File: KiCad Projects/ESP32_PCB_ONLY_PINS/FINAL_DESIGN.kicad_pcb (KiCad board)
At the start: 2 copper layers, 78 x 94.8 mm, 68 parts, among them J1 Screw_Terminal_01x02, J2 Conn_01x19_Socket, J3 Conn_01x19_Socket, J4 Conn_01x19_Socket, J5 Conn_01x19_Socket, Q1 PMOS, U1 LM2596S-5, U2 ESP32_NODEMCU

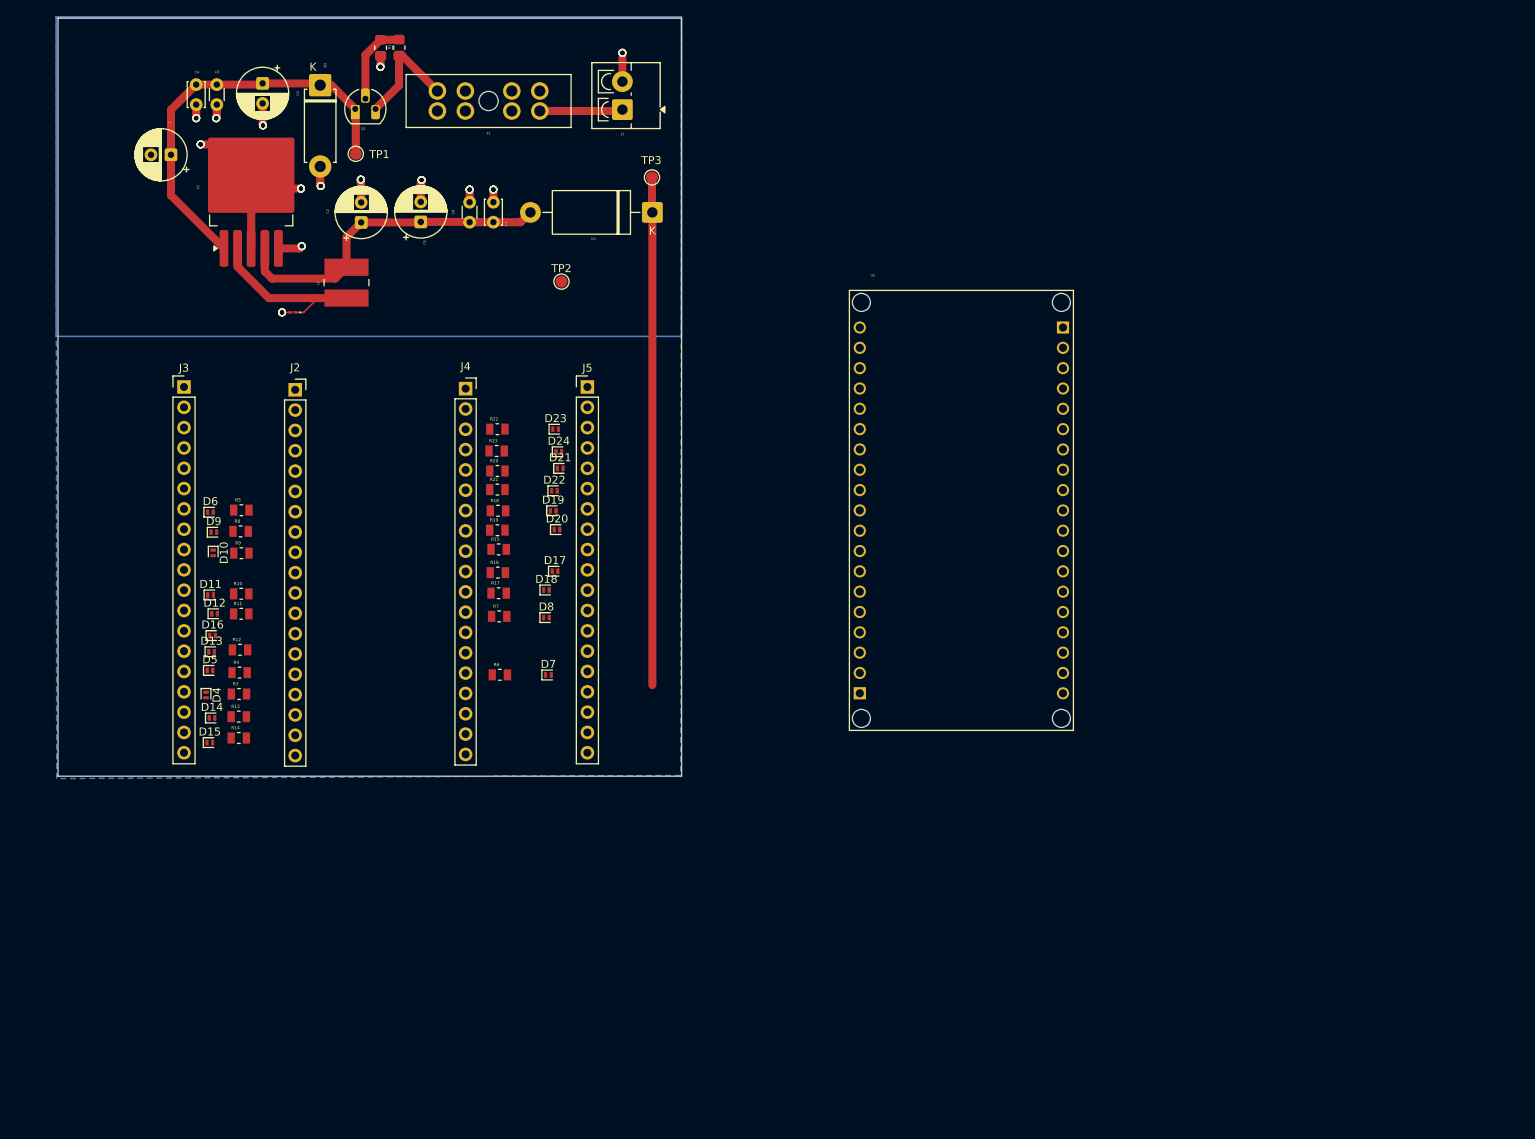
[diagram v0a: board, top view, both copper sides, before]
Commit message: PCB MODIFIED INSIDE ONLYPINS
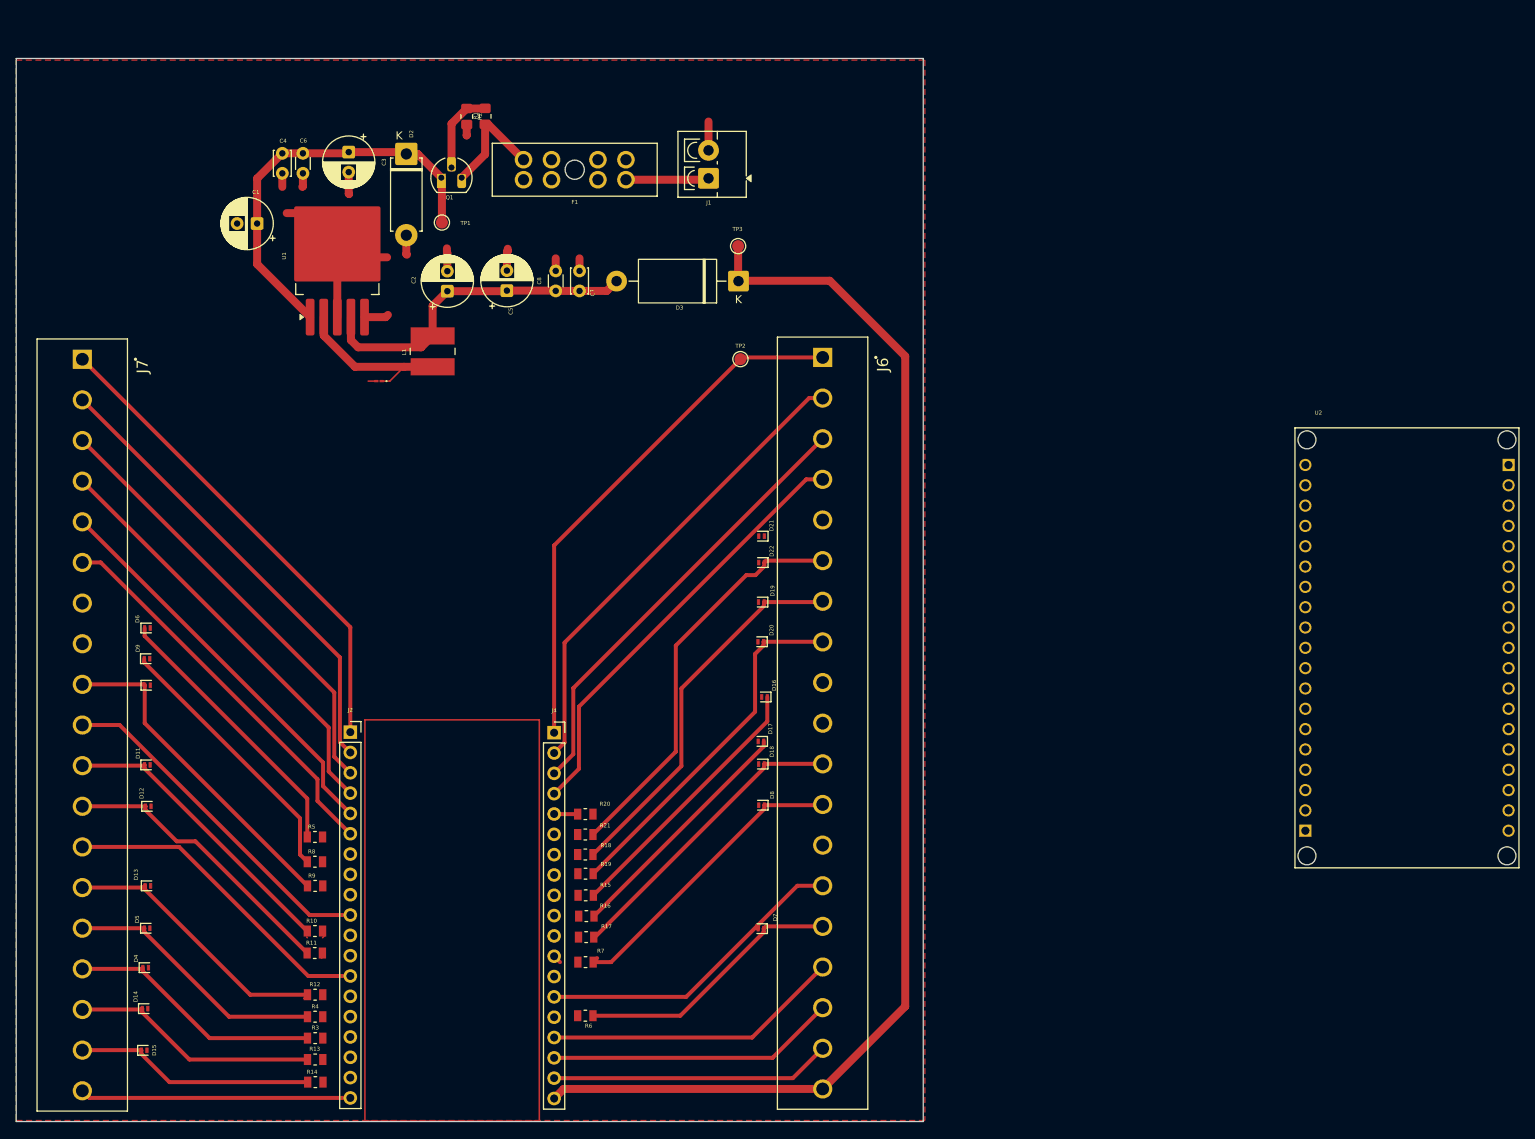
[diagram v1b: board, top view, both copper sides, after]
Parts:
- removed D23, D24: D_Zener, Diode_SMD:D_SOD-882
- removed J3, J5: Conn_01x19_Socket, Connector_PinHeader_2.54mm:PinHeader_1x19_P2.54mm_Vertical
- removed R22, R23: 100, RC0805FR-07330RL:RESC2012X60N
- added J6: TB010-508-P19BK, TB010-508-P19BK:CUI_TB010-508-P19BK, F.Cu at (163.2, 69.9)
- added J7: TB010-508-P19BK, TB010-508-P19BK:CUI_TB010-508-P19BK, F.Cu at (70.6, 70.1)
- moved D16 69.4 mm to (155.9, 112.3), turned to 180 degrees
- moved U2 58.3 mm to (236.2, 106.2)
- moved R15 44.6 mm to (133.5, 137.1), turned to 180 degrees
- moved R7 44.5 mm to (133.5, 145.5), turned to 180 degrees
- moved R21 44.5 mm to (133.5, 129.5), turned to 180 degrees
- moved J4 44.4 mm to (129.6, 116.8)
- moved R17 44.4 mm to (133.6, 142.3), turned to 180 degrees
- moved R16 44.3 mm to (133.6, 139.7), turned to 180 degrees
- moved R19 44.3 mm to (133.5, 134.4), turned to 180 degrees
- moved R18 44.3 mm to (133.5, 132.0), turned to 180 degrees
- moved R20 44.3 mm to (133.5, 127.0), turned to 180 degrees
- moved R12 44.1 mm to (99.7, 149.5)
- moved R14 44.1 mm to (99.7, 160.5)
- moved R3 44.1 mm to (99.7, 155.0)
- moved R4 44.0 mm to (99.7, 152.3)
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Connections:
- J2 pad 1: /IO_6 -> /CLK
- J2 pad 10: /IO_5 -> /I/O_5
- J2 pad 2: /IO_7 -> /SD0
- J2 pad 3: /IO_8 -> /SD1
- J2 pad 4: /IO_15 -> /I/O_15
- J2 pad 5: /IO_2 -> /I/O_2
- J2 pad 6: /IO_0 -> /I/O_0
- J4 pad 13: /IO_12 -> /I/O_12
- J4 pad 16: /IO_9 -> /SD2
- J4 pad 17: /IO_10 -> /SD3
- J4 pad 18: /IO_11 -> /CMD
- J4 pad 3: /IO_36 -> /SP
- J4 pad 4: /IO_39 -> /SN
- R8 pad 2: /IO16 -> /IO_16
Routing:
- net GND: track 50.5 -> 164.2 mm, vias 56 -> 0
- net VIN 5V: track 63.5 -> 159.1 mm
- net +3V3: track 0.00 -> 66.7 mm
- net /CLK: track 0.00 -> 60.8 mm
- net /EN: track 0.00 -> 59.3 mm
- net /SD0: track 0.00 -> 58.3 mm
- net /SD1: track 0.00 -> 55.8 mm
- net /SP: track 0.00 -> 55.7 mm
- net /SN: track 0.00 -> 54.6 mm
- net /I/O_15: track 0.00 -> 53.2 mm
- net /I/O_35: track 0.00 -> 50.9 mm
- net /I/O_2: track 0.00 -> 50.7 mm
- net /I/O_0: track 0.00 -> 49.5 mm
- net /I/O_32: track 0.00 -> 47.8 mm
- net /I/O_33: track 0.00 -> 45.2 mm
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- added copper zone on F.Cu, net GND
- removed copper zone on B.Cu, net GND
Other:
- board size 78 x 94.8 mm -> 113.4 x 132.9 mm

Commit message: PCB CHANGE
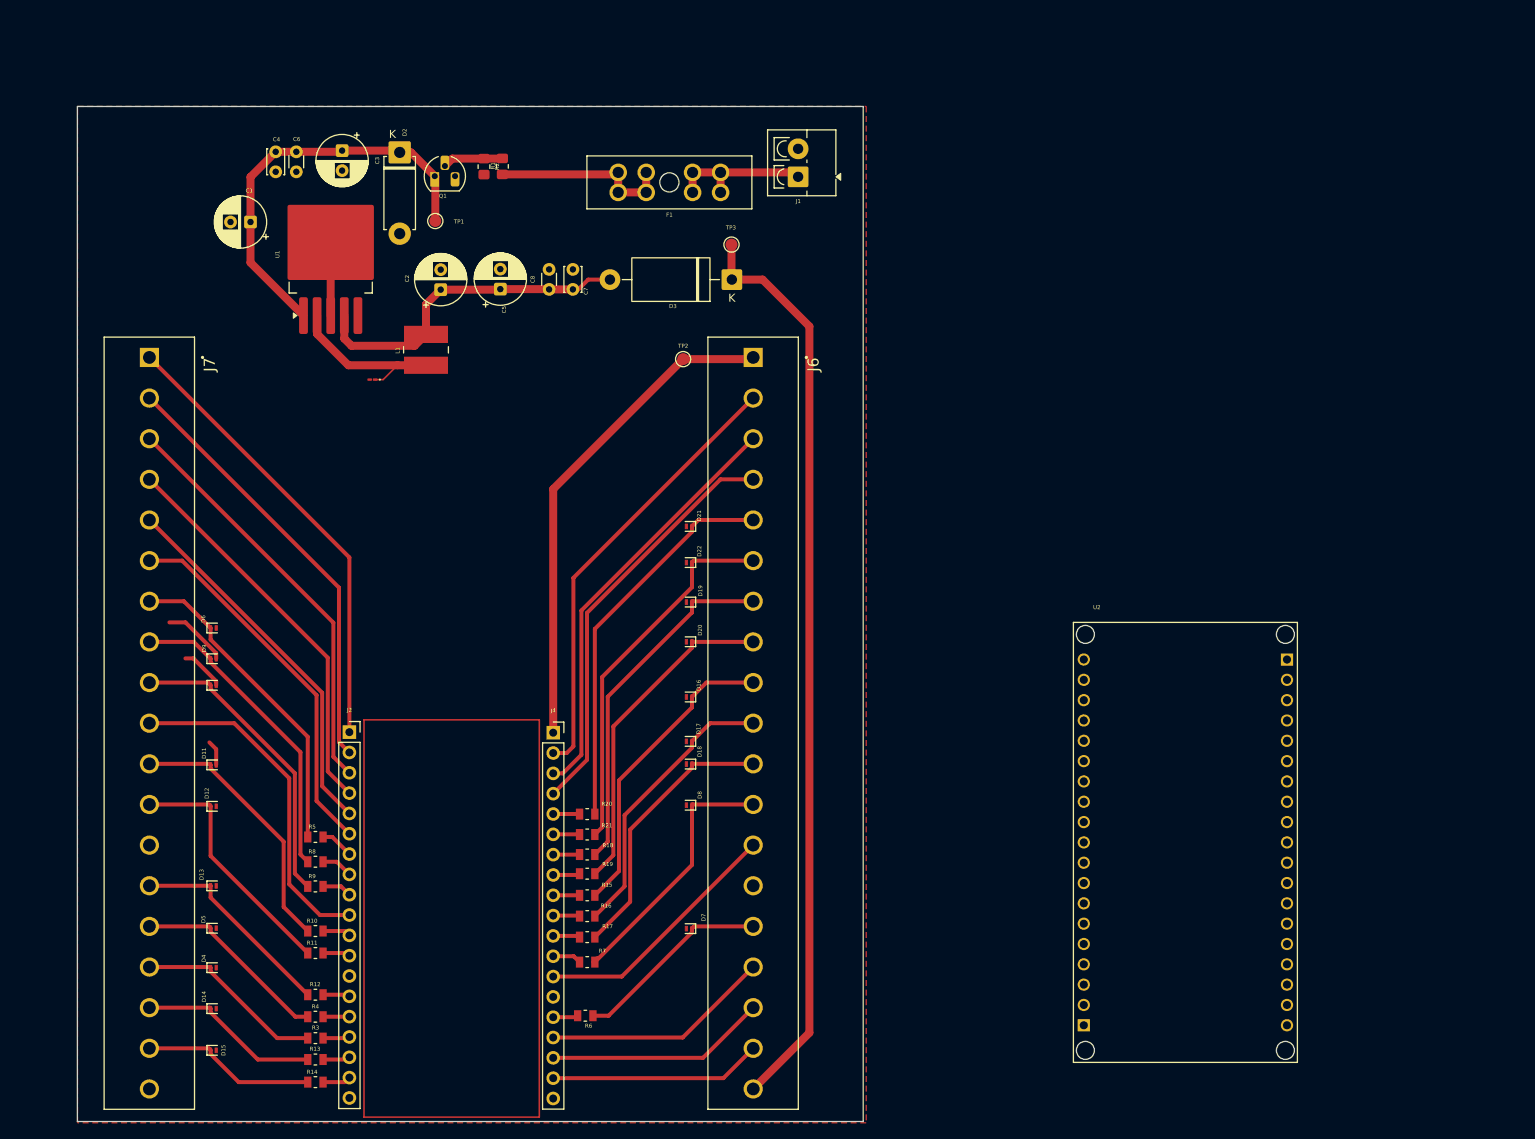
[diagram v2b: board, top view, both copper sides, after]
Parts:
- moved U2 36.9 mm to (208.5, 130.5)
- moved F1 11.9 mm to (150.4, 49.2)
- moved J1 11.2 mm to (160.1, 47.3)
- moved D16 9.41 mm to (146.5, 112.3)
- moved D21 9.12 mm to (146.5, 91.0)
- moved D8 9.05 mm to (146.5, 125.9)
- moved D22 9.04 mm to (146.5, 95.5)
- moved D18 9.03 mm to (146.5, 120.7)
- moved D19 9.02 mm to (146.5, 100.5)
- moved D17 8.97 mm to (146.5, 117.9)
- moved D7 8.96 mm to (146.5, 141.3)
- moved D20 8.94 mm to (146.5, 105.4)
- moved J6 8.69 mm to (154.5, 69.9)
- moved D15 8.66 mm to (87.0, 156.5)
- moved D14 8.55 mm to (87.0, 151.3)
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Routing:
- net GND: track 164.2 -> 33.8 mm
- net /I/O_34: track 0.07 -> 49.0 mm
- net VIN 5V: track 159.1 -> 114.7 mm
- net /I/O_12: track 0.00 -> 31.8 mm
- net /I/O_21: track 35.1 -> 26.3 mm
- net /I/O_13: track 33.6 -> 24.9 mm
- net /RXD: track 33.3 -> 24.7 mm
- net /SD2: track 37.2 -> 28.6 mm
- net /CMD: track 35.1 -> 26.5 mm
- net /SD3: track 36.2 -> 27.6 mm
- net Net-(Q1-S): track 14.5 -> 23.1 mm
- net /TXD: track 32.3 -> 23.8 mm
- net /I/O_22: track 31.2 -> 22.7 mm
- net /I/O_23: track 30.1 -> 21.8 mm
- net Net-(J1-Pin_1): track 10.6 -> 18.4 mm
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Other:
- board size 113.4 x 132.9 mm -> 98.2 x 126.9 mm
